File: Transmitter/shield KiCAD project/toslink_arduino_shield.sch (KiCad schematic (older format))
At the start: 21 parts, among them J1 solder_bridge, J2 solder_bridge, J3 solder_bridge, J4 solder_bridge, J5 solder_bridge, J6 solder_bridge, J7 solder_bridge, J8 solder_bridge, J9 solder_bridge, P1 Arduino UNO, P2 Toslink CNC Transciever, P3 PoStep25-32_connector, P4 PoStep25-32_connector, P5 PoStep25-32_connector, P6 CONN_01X04, P7 CONN_01X04, U1 SN74LV21APWR

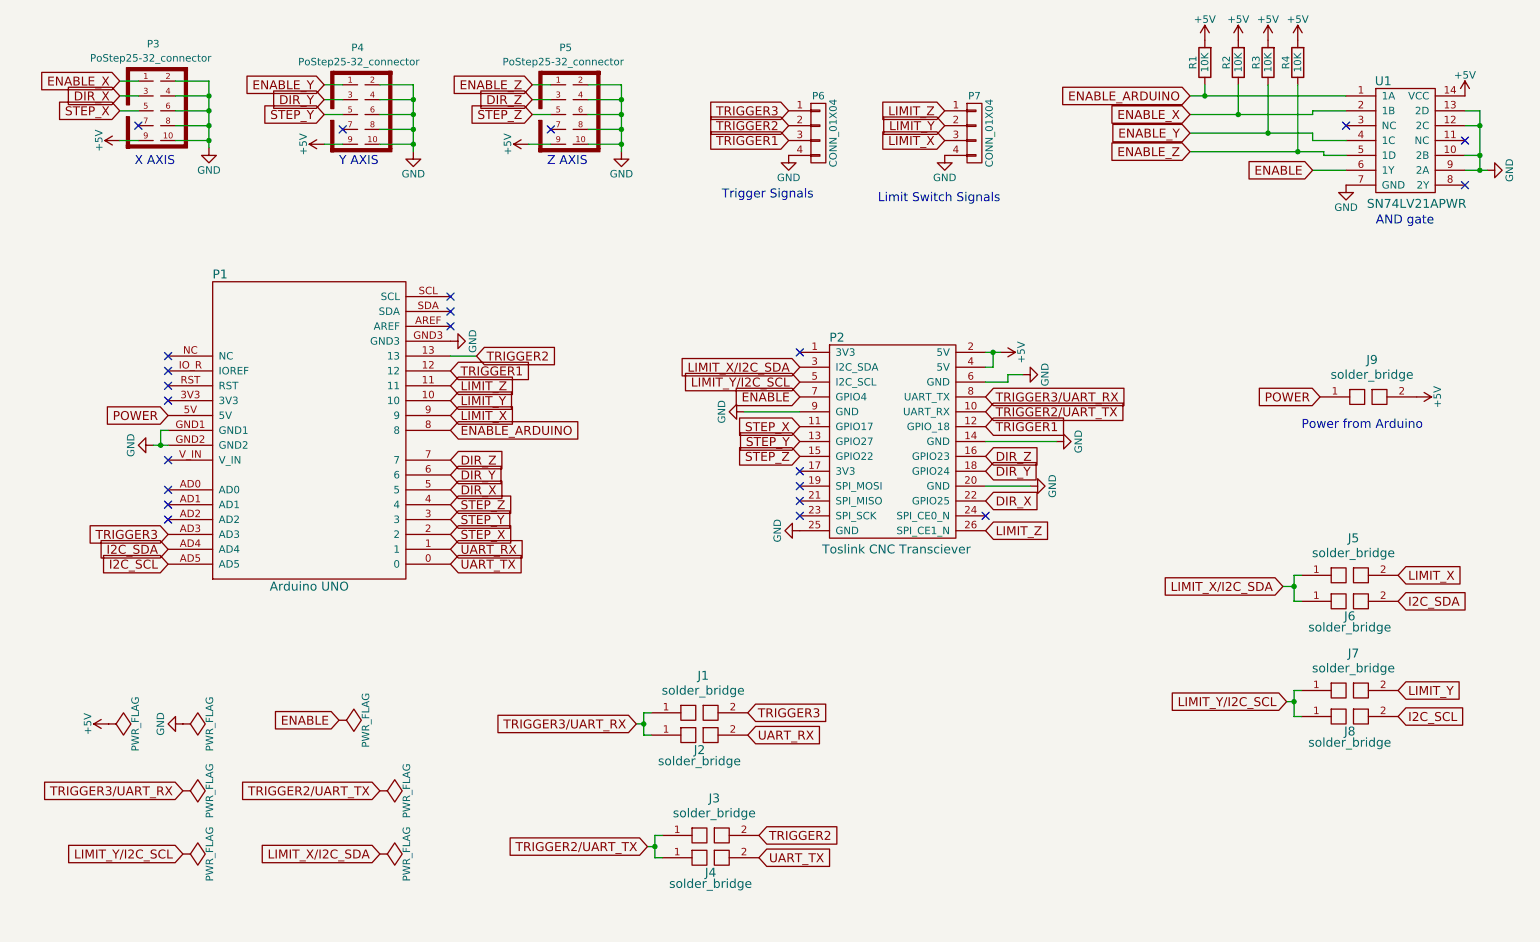
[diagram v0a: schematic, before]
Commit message: Update
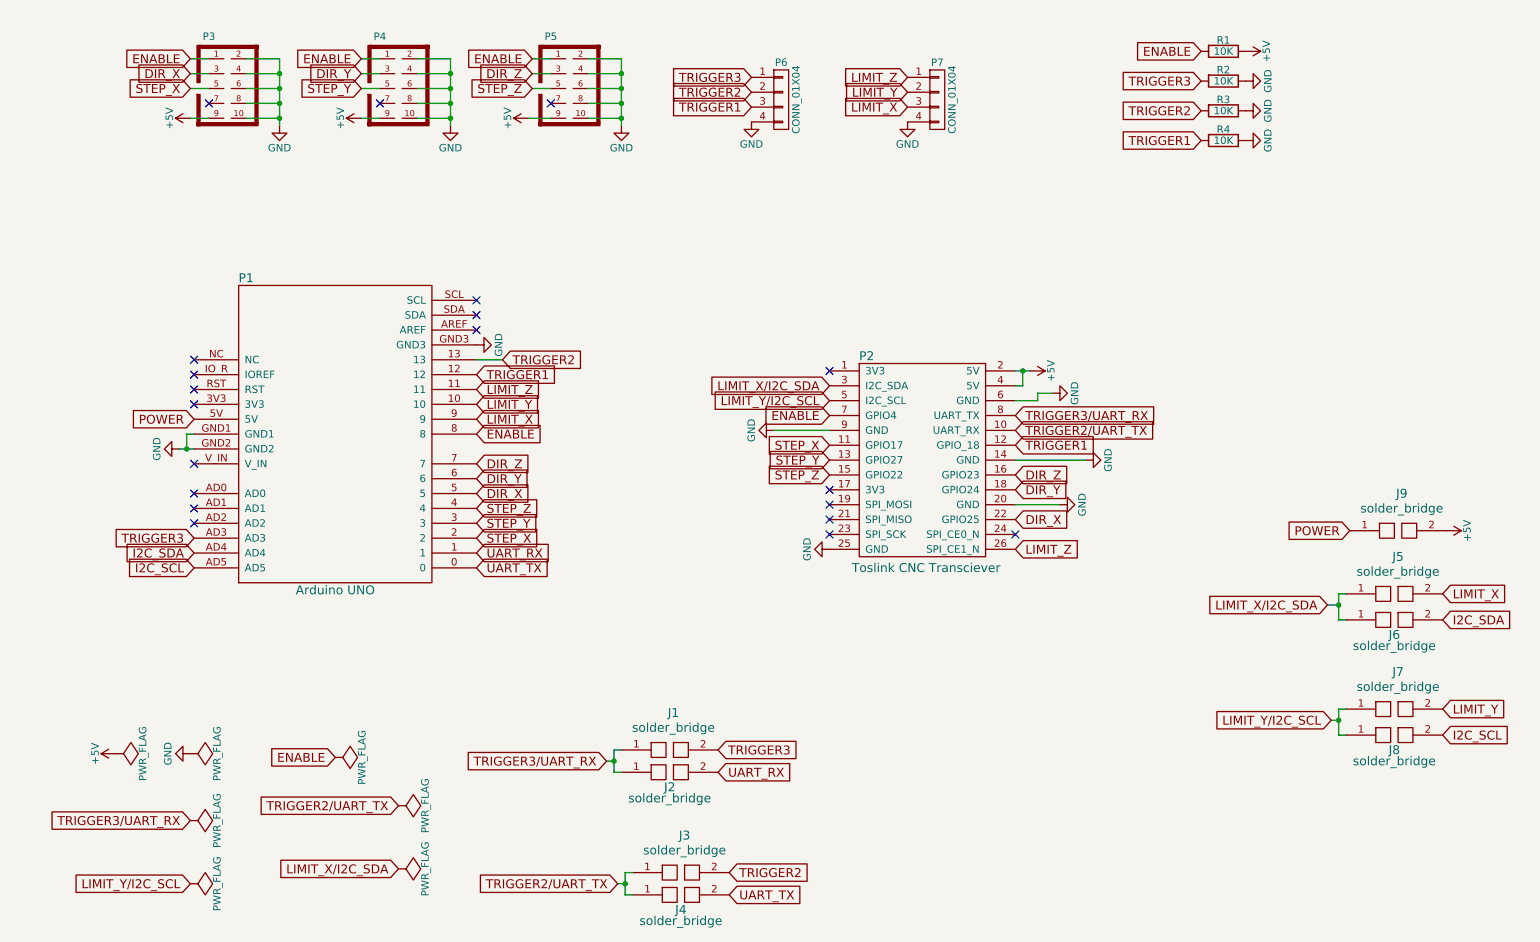
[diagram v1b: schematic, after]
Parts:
- removed U1: SN74LV21APWR, SN74LV21APWR_ANDGate:SN74LV21APWR_ANDGate_tssop14, symbol SN74LV21APWR__AND_Gate
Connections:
- net +5V: now also R1.1; no longer R1.2, R2.2, R3.2, R4.2
- net ENABLE: now also P1.8, P3.1, P4.1, P5.1, R1.2
- net GND: now also R2.1, R3.1, R4.1
- net TRIGGER1: now also R4.2
- net TRIGGER2: now also R3.2
- net TRIGGER3: now also R2.2
- removed net ENABLE_ARDUINO: P1.8, R1.1
- removed net ENABLE_X: P3.1, R2.1
- removed net ENABLE_Y: P4.1, R3.1
- removed net ENABLE_Z: P5.1, R4.1
- no-connect marks 23 -> 20
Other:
- note removed: "AND gate"
- note removed: "Limit Switch Signals"
- note removed: "Power from Arduino"
- note removed: "Trigger Signals"
- note removed: "X AXIS"
- note removed: "Y AXIS"
- note removed: "Z AXIS"
- moved on the sheet: J1, J2, J3, J4, J5, J6, J7, J8, J9, P1, P2, P3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
